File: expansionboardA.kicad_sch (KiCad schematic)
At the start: 40 parts, among them J1 DEBUG, J2 USB_A_Stacked, J3 HDMI_A, P1 USB_C_Plug, U1 MAX3420EECJ, U2 GPIO_U2, U3 AMS1117-3.3, U4 GPIO_U4, U5 MCP3008T-I/SL, U6 TLV320AIC23BIPW, Y1 Crystal

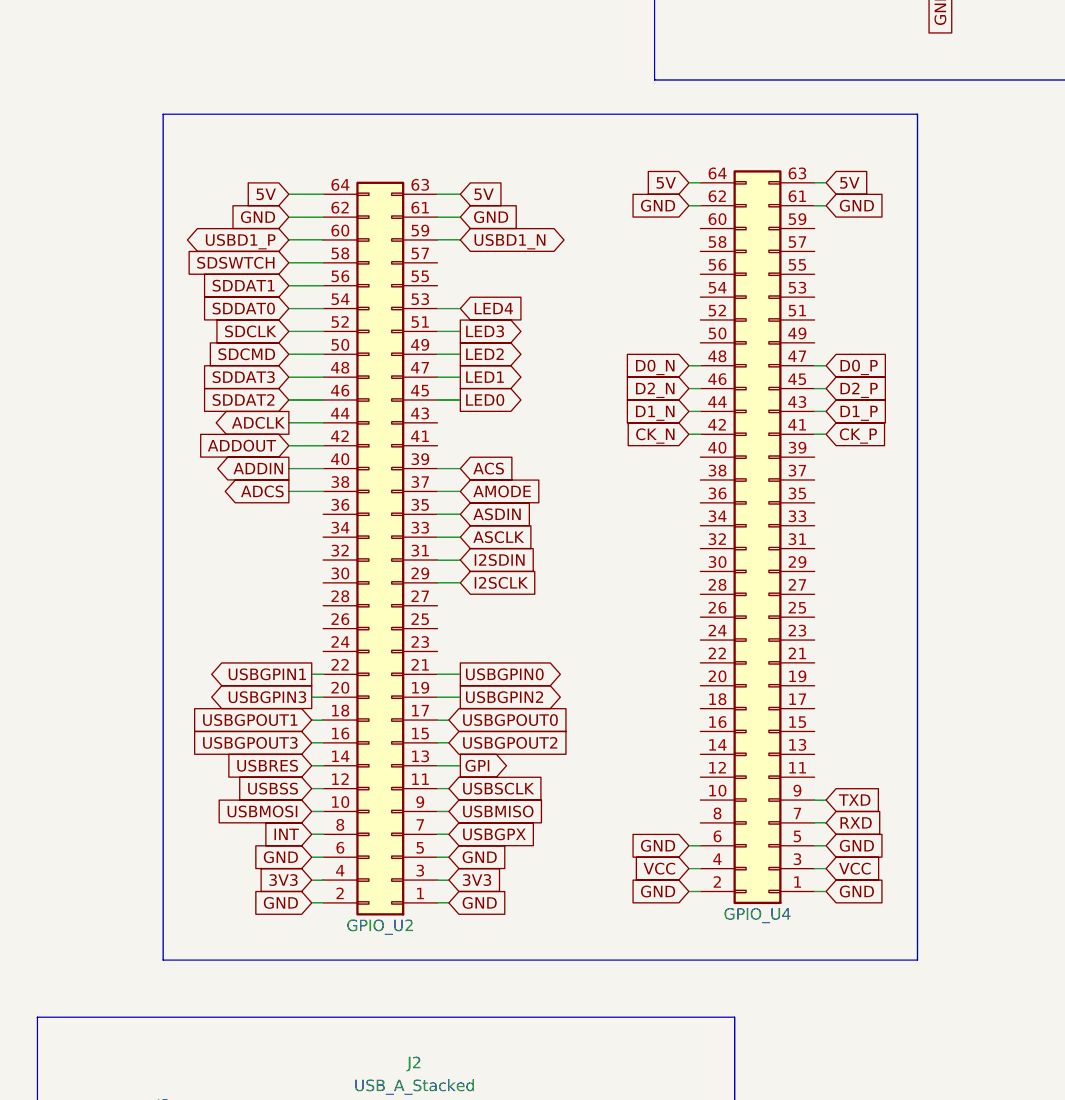
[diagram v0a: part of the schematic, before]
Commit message: Updated board
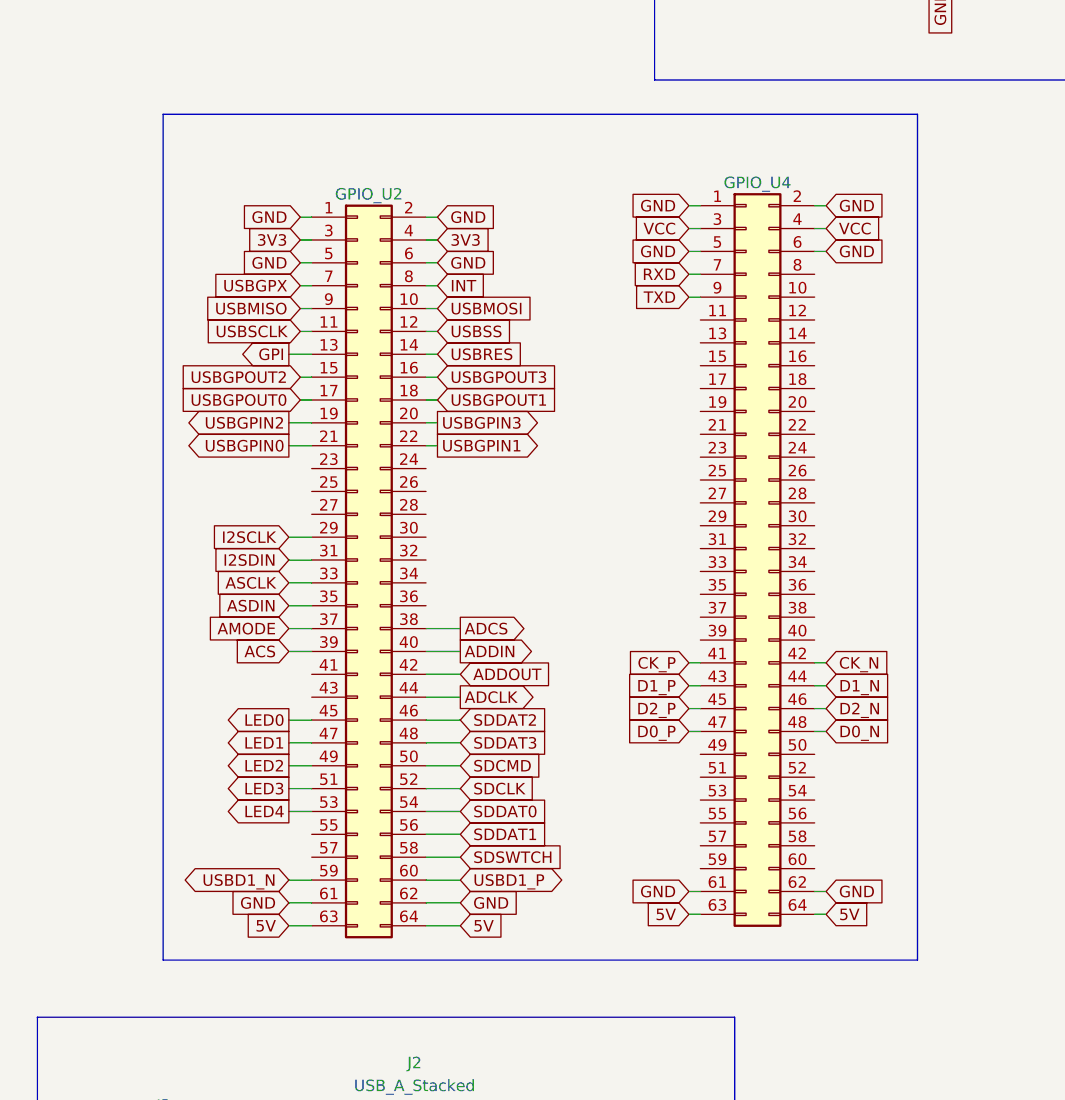
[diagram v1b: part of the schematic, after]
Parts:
- C1, C2, C3, C4, C5: footprint Capacitor_SMD:C_0603_1608Metric -> Capacitor_SMD:C_0603_1608Metric_Pad1.08x0.95mm_HandSolder
- R1, R10, R2, R3, R4, R5, R6, R7, R9: footprint Resistor_SMD:R_0603_1608Metric -> Resistor_SMD:R_0603_1608Metric_Pad0.98x0.95mm_HandSolder
- U3: footprint Package_TO_SOT_SMD:SOT-89-3 -> Package_TO_SOT_SMD:SOT-89-3_Handsoldering

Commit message: Updatre board version
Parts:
- removed AU2: SJ-3523-SMT-TR, SJ-3523-SMT-TR:CUI_SJ-3523-SMT-TR, symbol SJ-3523-SMT-TR:SJ-3523-SMT-TR
- removed D6: LED, LED_SMD:LED_1206_3216Metric_Pad1.42x1.75mm_HandSolder, symbol Device:LED
- removed U6: TLV320AIC23BIPW, TLV320AIC23BIPW:SOP65P640X120-28N, symbol TLV320AIC23BIPW:TLV320AIC23BIPW
- added C10: 0.1uf, Capacitor_SMD:C_0603_1608Metric_Pad1.08x0.95mm_HandSolder, symbol Device:C
- added C11, C13, C14: 3.3uf, Capacitor_THT:CP_Radial_D5.0mm_P2.50mm, symbol Device:C_Polarized_US
- added C12: 10uf, Capacitor_THT:CP_Radial_D5.0mm_P2.50mm, symbol Device:C_Polarized_US
- added C8, C9: 1uf ceramic, Capacitor_SMD:C_0603_1608Metric_Pad1.08x0.95mm_HandSolder, symbol Device:C
- added R11, R14: 10KOhm, Resistor_SMD:R_0603_1608Metric_Pad0.98x0.95mm_HandSolder, symbol Device:R
- added R12, R13: 470Ohm, Resistor_SMD:R_0603_1608Metric_Pad0.98x0.95mm_HandSolder, symbol Device:R
- added R8: R33_ohm, Resistor_SMD:R_0603_1608Metric_Pad0.98x0.95mm_HandSolder, symbol Device:R
- added U6: CS4344-CZZR, CIR_3TSSOP-10, symbol 2023-04-16_23-08-01:CS4344-CZZR
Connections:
- net HPOUTLEFT is gone; now on an unnamed net: AU1.3
- net GND: now also C10.2, C11.2, C12.2, C8.1, C9.2, R11.2, R14.2, U6.8 (GND)
- net at R7.2: now also C8.2
- net ACS: no longer names the net of U2.39 (Pin_39)
- net AMODE: no longer names the net of U2.37 (Pin_37)
- net ASCLK renamed AU_LRCLK
- net AU_LRCLK: now also U6.3 (LRCK)
- net ASDIN renamed AU_MCLK
- net AU_MCLK: now also U6.4 (MCLK)
- net HPOUTRIGHT: no longer names the net of AU1.2
- net HPOUTRIGHT: now also C9.1, R8.2
- net I2SCLK renamed AU_SDIN
- net AU_SDIN: now also U6.1 (SDIN)
- net I2SDIN renamed AU_SCLK
- net AU_SCLK: now also U6.2 (*DEM/SCLK)
- net LED4: no longer names the net of U2.53 (Pin_53)
- net LED4: no longer R7.1
- new net: C13.2, R11.1, R12.1
- new net: C14.2, R13.1, R14.1
- new net: C12.1, U6.6 (FILT+)
- new net: C10.1, C11.1, U6.5 (VQ)
- new net AL: C14.1, U6.7 (AOUTL)
- new net AR: C13.1, U6.10 (AOUTR)
- new net LEFTOUT: R13.2, R7.1
- new net RIGHTOUT: R12.2, R8.1
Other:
- note added: "3v3 Power Regulator"
- note added: "Analog / Digital converter"
- note added: "Audio Out"
- note added: "Audio Output"
- note added: "DVI out over HDMI"
- note added: "Debug LEDs"
- note added: "FPGA board GPIO pins"
- note added: "Micro SD Card"
- note added: "Serial Debug Port"
- note added: "USB-A Host socket"
- note added: "USB-C Power and Data"
- moved on the sheet: ADC1, AU1, C1, C2, C3, C4, C5, C6, C7, CRD1, D1, D2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
